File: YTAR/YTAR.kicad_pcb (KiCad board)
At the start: 6 copper layers, 50 x 50 mm, 223 parts, among them J1 STDC14, J2 CAMERA, J3 Micro_Sd, J4 FH12-40S-0.5SH(55), J5 USB_C_USB4085-GF-A, J6 IO, SW1 RESET, SW2 PICTURE, SW3 MODE, U1 STM32H750XBHx, U2 MCP2562-E-MF, U3 DS90C124, U5 TPS56339, U6 TPS56339, Y1 25MHz

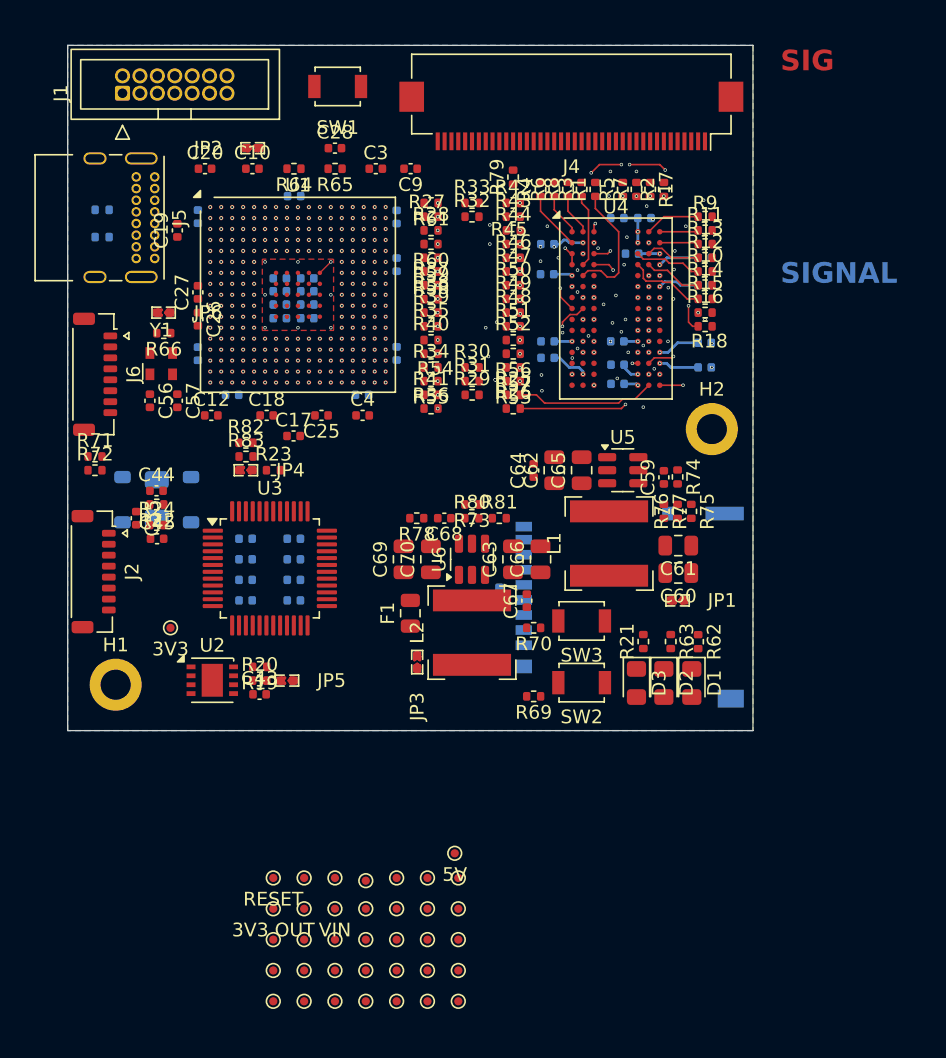
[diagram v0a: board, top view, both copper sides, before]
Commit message: routing checkpoint
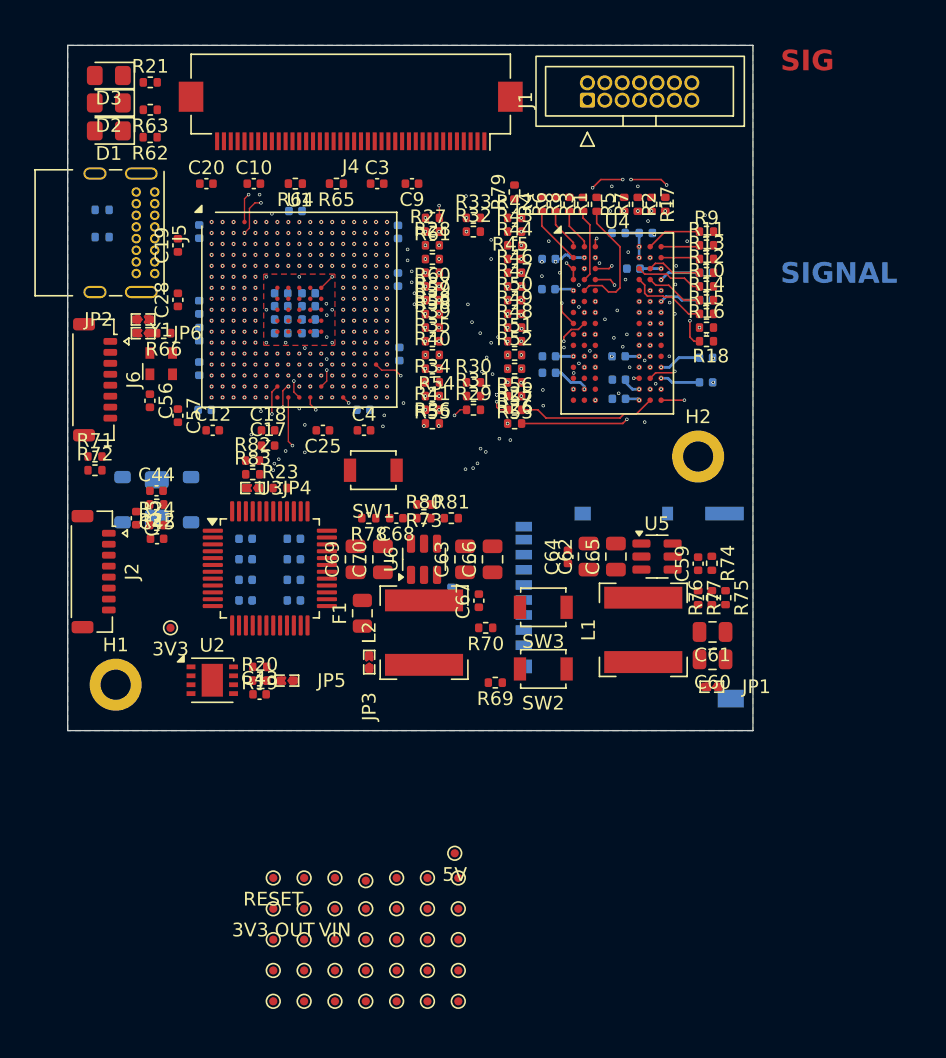
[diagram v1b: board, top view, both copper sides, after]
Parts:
- C26, C27: moved to B.Cu
- moved D3 58.7 mm to (15.0, 14.2), turned to 180 degrees
- moved D1 58.6 mm to (15.0, 18.2), turned to 180 degrees
- moved D2 58.6 mm to (15.0, 16.2), turned to 180 degrees
- moved R21 54.4 mm to (18.0, 14.7), turned to 0 degrees
- moved R62 54.3 mm to (18.0, 18.7), turned to 180 degrees
- moved R63 54.3 mm to (18.0, 16.7), turned to 180 degrees
- moved J1 33.9 mm to (49.9, 16.0)
- moved SW1 28.1 mm to (34.3, 43.0)
- moved J4 16.1 mm to (32.6, 17.1)
- moved C28 15.9 mm to (20.0, 30.6), turned to 90 degrees
- moved JP2 14.8 mm to (17.5, 32.0)
- moved C59 6.78 mm to (58.0, 49.8)
- moved C60 6.78 mm to (59.0, 56.8)
- moved C61 6.78 mm to (59.0, 54.8)
- moved C62 6.78 mm to (50.0, 49.3)
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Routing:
- net Net-(U1-PF13): track 0.00 -> 38.1 mm, vias 1 -> 6
- net Net-(U1-PF12): track 0.00 -> 35.7 mm, vias 1 -> 5
- net Net-(U1-PF11): track 0.00 -> 32.7 mm, vias 1 -> 5
- net Net-(U1-PF15): track 0.00 -> 28.0 mm, vias 1 -> 6
- net Net-(U1-PE0): track 0.00 -> 27.2 mm, vias 1 -> 4
- net Net-(U1-PG0): track 0.00 -> 27.1 mm, vias 1 -> 6
- net Net-(U1-PH5): track 0.00 -> 26.6 mm, vias 1 -> 4
- net Net-(U1-PG1): track 0.00 -> 24.3 mm, vias 1 -> 3
- net Net-(U1-PE1): track 0.00 -> 18.4 mm, vias 1 -> 3
- net Net-(U1-PG15): track 0.00 -> 14.6 mm, vias 1 -> 3
- net Net-(U1-PD15): track 0.00 -> 14.4 mm, vias 1 -> 3
- net Net-(U1-PE9): track 0.00 -> 13.7 mm, vias 1 -> 3
- net Net-(U1-PE10): track 0.00 -> 12.6 mm, vias 1 -> 4
- net Net-(U1-PD14): track 0.00 -> 12.6 mm, vias 1 -> 3
- net Net-(U1-PE8): track 0.00 -> 12.0 mm, vias 1 -> 3
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
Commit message: DRAM routed
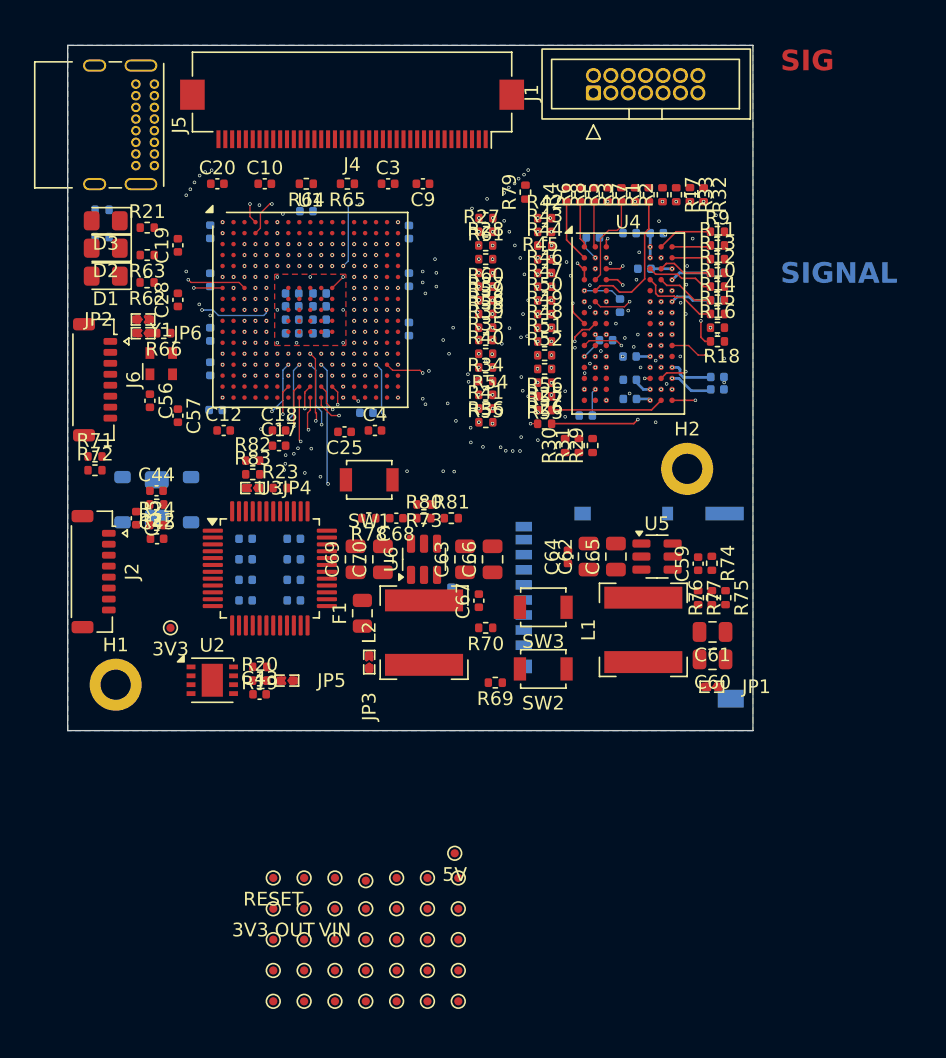
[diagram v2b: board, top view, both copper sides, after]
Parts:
- moved R32 17.0 mm to (58.4, 22.9), turned to -90 degrees
- moved R33 15.9 mm to (57.4, 22.9), turned to -90 degrees
- moved D1 10.6 mm to (14.8, 28.8)
- moved D2 10.6 mm to (14.8, 26.8)
- moved D3 10.6 mm to (14.8, 24.8)
- moved R21 10.6 mm to (17.8, 25.3)
- moved R62 10.6 mm to (17.8, 29.3)
- moved R63 10.6 mm to (17.8, 27.3)
- moved R29 9.07 mm to (50.3, 41.2), turned to 90 degrees
- moved R31 8.50 mm to (49.3, 41.2), turned to 90 degrees
- moved R30 8.12 mm to (48.3, 41.2), turned to 90 degrees
- moved J5 7.88 mm to (18.3, 14.8)
- moved C37 5.36 mm to (52.3, 31.0), turned to -90 degrees
- moved C32 4.32 mm to (51.3, 33.5), turned to 0 degrees
- moved C40 4.11 mm to (49.8, 39.0)
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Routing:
- net Net-(U1-PF4): track 0.00 -> 47.1 mm, vias 1 -> 6
- net Net-(U1-PF5): track 0.00 -> 46.0 mm, vias 2 -> 5
- net Net-(U1-PF3): track 0.00 -> 44.4 mm, vias 1 -> 6
- net Net-(U1-PF1): track 0.00 -> 39.8 mm, vias 1 -> 5
- net Net-(U1-PF2): track 0.00 -> 39.7 mm, vias 1 -> 5
- net Net-(U1-PF0): track 0.00 -> 39.1 mm, vias 1 -> 6
- net Net-(U1-PF14): track 0.00 -> 32.7 mm, vias 2 -> 6
- net Net-(U1-PE0): track 27.2 -> 2.96 mm, vias 4 -> 3
- net /NBL1: track 0.00 -> 20.4 mm, vias 0 -> 2
- net Net-(U1-PE11): track 11.3 -> 31.1 mm, vias 3 -> 5
- net Net-(U1-PE12): track 10.8 -> 30.2 mm, vias 3 -> 5
- net Net-(U1-PE1): track 18.4 -> 2.72 mm, vias 3 -> 1
- net Net-(U1-PE8): track 12.0 -> 27.5 mm, vias 3 -> 5
- net /NBL0: track 0.00 -> 14.1 mm, vias 0 -> 2
- net Net-(U1-PE10): track 12.6 -> 25.3 mm, vias 4 -> 5
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
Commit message: DRAM routed hmm
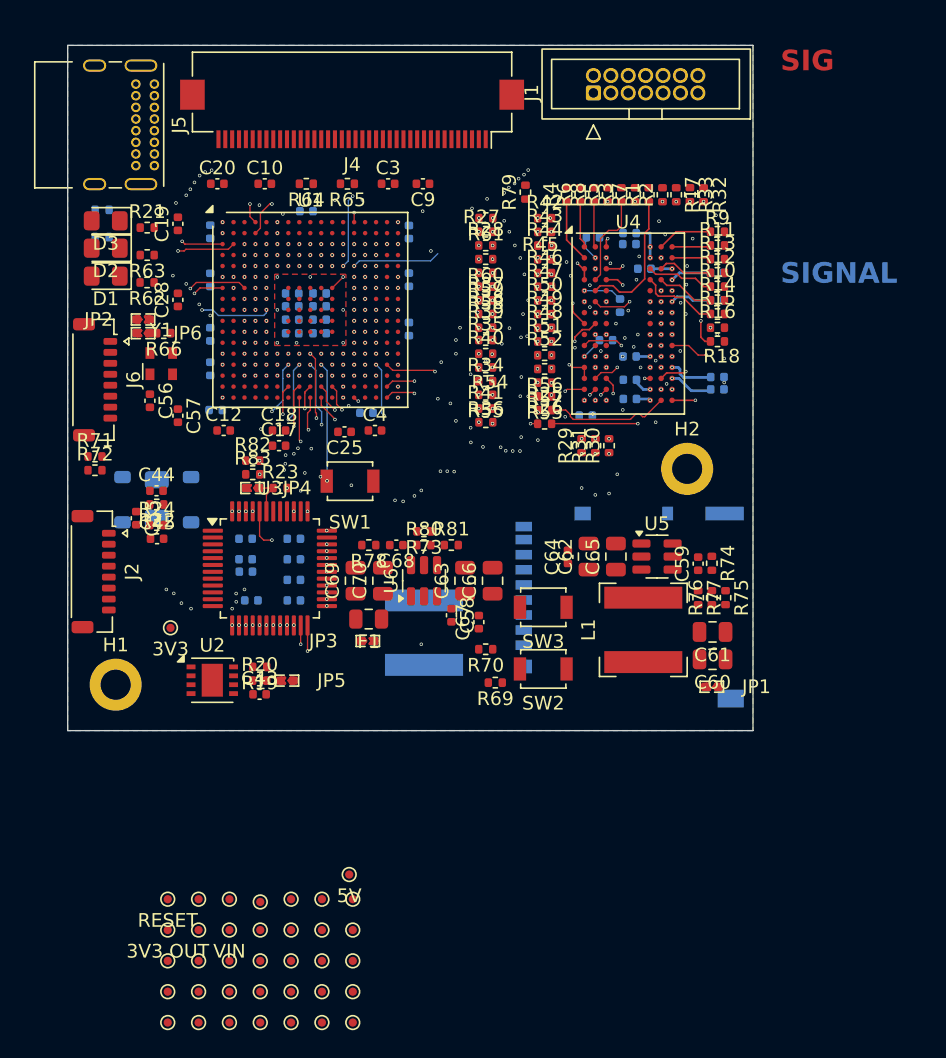
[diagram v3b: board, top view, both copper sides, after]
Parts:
- C58: moved to F.Cu
- L2: moved to B.Cu
- moved TP12 7.85 mm to (32.5, 72.5)
- moved TP33 7.85 mm to (32.8, 74.3)
- moved TP34 7.85 mm to (32.8, 76.5)
- moved TP35 7.85 mm to (32.8, 78.8)
- moved TP36 7.85 mm to (32.8, 81.0)
- moved TP37 7.85 mm to (32.8, 83.3)
- moved TP1 7.85 mm to (19.3, 74.3)
- moved TP10 7.85 mm to (21.6, 83.3)
- moved TP11 7.85 mm to (23.8, 74.3)
- moved TP14 7.85 mm to (23.8, 76.5)
- moved TP15 7.85 mm to (23.8, 78.8)
- moved TP16 7.85 mm to (23.8, 81.0)
- moved TP17 7.85 mm to (23.8, 83.3)
- moved TP18 7.85 mm to (26.1, 74.5)
- moved TP19 7.85 mm to (26.1, 76.5)
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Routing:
- net /ROUT12: track 0.00 -> 52.6 mm, vias 1 -> 6
- net /ROUT10: track 0.00 -> 45.1 mm, vias 0 -> 5
- net /ROUT9: track 0.00 -> 44.4 mm, vias 1 -> 4
- net /DQ12: track 0.00 -> 38.5 mm, vias 1 -> 5
- net /ROUT14: track 0.00 -> 36.0 mm, vias 0 -> 4
- net /ROUT13: track 0.00 -> 36.0 mm, vias 1 -> 5
- net /ROUT15: track 0.00 -> 34.4 mm, vias 0 -> 4
- net Net-(U1-PD10): track 0.00 -> 28.7 mm, vias 0 -> 4
- net Net-(U1-PD9): track 0.00 -> 28.2 mm, vias 0 -> 4
- net Net-(U1-PD8): track 0.00 -> 24.9 mm, vias 0 -> 4
- net /DES_RCLK: track 0.00 -> 12.2 mm, vias 0 -> 2
- net /DES_LOCK: track 0.00 -> 11.0 mm, vias 0 -> 2
- net /ROUT8: track 0.00 -> 8.35 mm, vias 1 -> 2
- net GND: track 3.24 -> 8.61 mm, vias 47 -> 51
- net /DQ14: track 0.00 -> 4.73 mm, vias 0 -> 2
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
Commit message: Huuuh
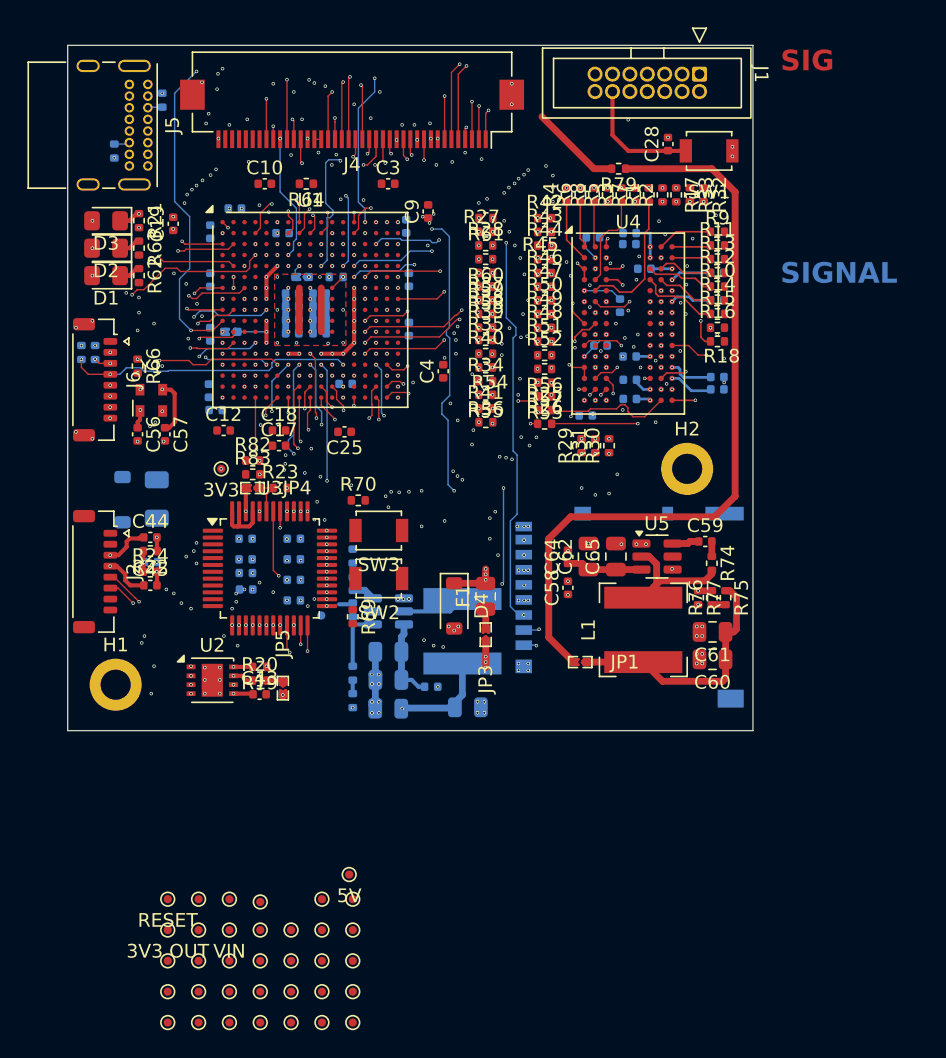
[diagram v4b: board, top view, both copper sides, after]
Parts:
- C20, C55, C63, C66, C67, C68, C69, C70, JP2, JP6, R65, R71, R72, R73, R78, R80, R81, TP23, U6: moved to B.Cu
- D4: moved to F.Cu
- moved C28 37.5 mm to (55.8, 19.2)
- moved SW1 35.6 mm to (58.8, 19.7)
- moved TP23 20.8 mm to (30.5, 53.6), turned to 180 degrees
- moved D4 20.7 mm to (40.2, 52.9)
- moved R70 14.3 mm to (33.2, 45.2), turned to 0 degrees
- moved SW2 13.7 mm to (34.7, 50.9)
- moved R73 13.4 mm to (32.8, 59.8), turned to 90 degrees
- moved SW3 13.2 mm to (34.7, 47.4)
- moved TP13 12.2 mm to (23.2, 42.9)
- moved JP2 12.0 mm to (29.1, 28.9), turned to 0 degrees
- moved R69 11.5 mm to (32.8, 53.7), turned to -90 degrees
- moved C70 11.1 mm to (41.2, 60.3), turned to 0 degrees
- moved R80 10.7 mm to (32.8, 57.8), turned to 90 degrees
- moved C66 10.5 mm to (35.4, 58.3), turned to 180 degrees
- moved JP1 9.77 mm to (49.4, 57.0)
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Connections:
- JP5 pad 1: /CAN_L -> /CAM_CAN_L
- R20 pad 1: /CAN_H -> /CAM_CAN_H
- U1 pad B17: /FD_CAN1_RX -> unconnected-(U1-PH14-PadB17)
- U1 pad D5: unconnected-(U1-PB8-PadD5) -> /FD_CAN1_RX
- U1 pad R3: unconnected-(U1-PA6-PadR3) -> /IO_AUX_1
- U1 pad T3: unconnected-(U1-PA5-PadT3) -> /IO_AUX_2
- U2 pad 1: /CAN_TX -> /FD_CAN1_TX
- U2 pad 4: /CAN_RX -> /FD_CAN1_RX
- U2 pad 6: /CAN_L -> /CAM_CAN_L
- U2 pad 7: /CAN_H -> /CAM_CAN_H
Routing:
- net /~{STM_RST}: track 0.00 -> 64.8 mm, vias 0 -> 2
- net /LCD_R5: track 0.00 -> 64.3 mm, vias 0 -> 4
- net /SD_D3: track 0.00 -> 61.9 mm, vias 0 -> 4
- net /LCD_R4: track 0.00 -> 61.7 mm, vias 0 -> 4
- net /SD_D2: track 0.00 -> 60.9 mm, vias 0 -> 4
- net +5V: track 0.00 -> 55.5 mm, vias 0 -> 1
- net /ROUT11: track 0.00 -> 53.4 mm, vias 1 -> 4
- net /LCD_R1: track 0.00 -> 51.4 mm, vias 1 -> 4
- net /LCD_R2: track 0.00 -> 51.2 mm, vias 1 -> 4
- net /FD_CAN1_RX: track 0.00 -> 44.4 mm, vias 0 -> 4
- net /LCD_R0: track 0.00 -> 44.3 mm, vias 1 -> 4
- net /SD_CMD: track 0.00 -> 41.9 mm, vias 1 -> 3
- net /JTDO/SWO: track 0.00 -> 41.9 mm, vias 1 -> 2
- net /FD_CAN1_TX: track 0.00 -> 41.5 mm, vias 1 -> 4
- net /SD_CK: track 0.00 -> 40.8 mm, vias 0 -> 6
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- removed copper zone on B.Cu, net GND

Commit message: Trud skonczon
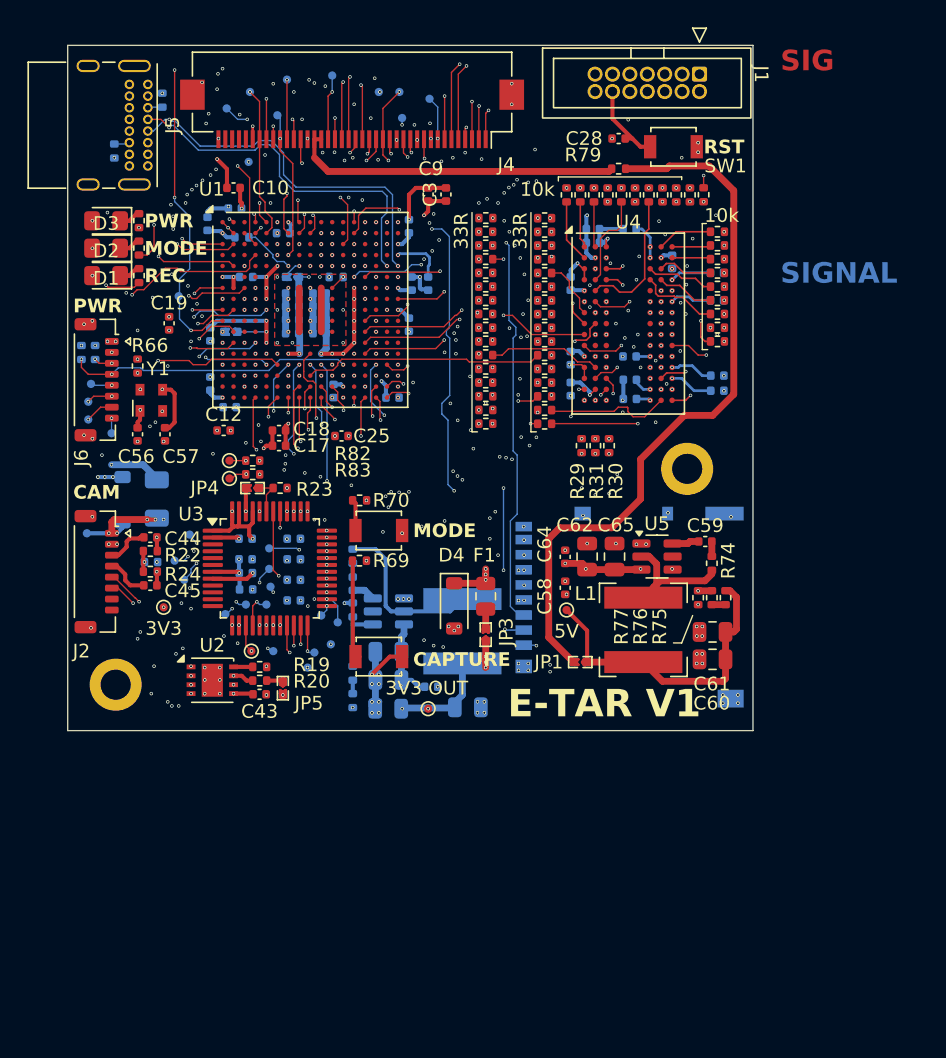
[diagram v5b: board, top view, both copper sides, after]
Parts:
- added C71: 2.2u, Capacitor_SMD:C_0402_1005Metric, B.Cu at (27.7, 25.7)
- C4, R64, TP1, TP10, TP11, TP14, TP15, TP16, TP17, TP18, TP19, TP20, TP21, TP22, TP24, TP25, TP26, TP27, TP28, TP3, TP30, TP31, TP34, TP35, TP36, TP37, TP4, TP5, TP6, TP7, TP8, TP9: moved to B.Cu
- moved TP5 70.1 mm to (31.3, 14.2), turned to 180 degrees
- moved TP4 67.8 mm to (36.2, 15.4), turned to 180 degrees
- moved TP10 67.6 mm to (36.4, 17.3), turned to 180 degrees
- moved TP3 65.7 mm to (38.4, 15.9), turned to 180 degrees
- moved TP8 64.6 mm to (28.0, 14.5), turned to 180 degrees
- moved TP9 64.2 mm to (27.3, 17.1), turned to 180 degrees
- moved TP15 63.4 mm to (25.3, 15.4), turned to 180 degrees
- moved TP7 60.0 mm to (23.6, 16.6), turned to 180 degrees
- moved TP11 59.9 mm to (34.7, 15.4), turned to 180 degrees
- moved TP6 53.9 mm to (25.2, 20.5), turned to 180 degrees
- moved TP37 46.5 mm to (15.2, 40.3), turned to 180 degrees
- moved TP36 46.0 mm to (13.5, 39.3), turned to 180 degrees
- moved TP35 45.1 mm to (13.5, 38.0), turned to 180 degrees
- moved TP34 44.2 mm to (13.7, 36.7), turned to 180 degrees
- moved TP1 44.0 mm to (20.1, 30.3), turned to 180 degrees
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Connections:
- net /IO_AUX_1 renamed /DCMI_PIXCLK
- C2 pad 1: Net-(C1-Pad1) -> Net-(C2-Pad1)
- U1 pad A2: unconnected-(U1-PI6-PadA2) -> /LED_ORANGE
- U1 pad A3: unconnected-(U1-PI5-PadA3) -> /DCMI_VSYNC
- U1 pad A4: unconnected-(U1-PI4-PadA4) -> /LED_GREEN
- U1 pad A5: unconnected-(U1-PB5-PadA5) -> /LCD_AUX_1
- U1 pad A7: Net-(C1-Pad1) -> Net-(C71-Pad1)
- U1 pad B16: unconnected-(U1-PH15-PadB16) -> /DCMI_D11
- U1 pad B17: unconnected-(U1-PH14-PadB17) -> /DCMI_D4
- U1 pad B5: unconnected-(U1-PB6-PadB5) -> /LCD_PWM
- U1 pad P13: unconnected-(U1-PH10-PadP13) -> /DCMI_D1
- U1 pad P14: unconnected-(U1-PH11-PadP14) -> /DCMI_D2
- U1 pad R14: unconnected-(U1-PH12-PadR14) -> /DCMI_D3
- U1 pad R15: unconnected-(U1-PD11-PadR15) -> /SD_DET_A
- U1 pad T14: unconnected-(U1-PB12-PadT14) -> /SW_MODE
- U1 pad U11: Net-(C1-Pad1) -> Net-(C2-Pad1)
- U1 pad U14: unconnected-(U1-PB13-PadU14) -> /SW_PICTURE
- U1 pad U3: unconnected-(U1-PA4-PadU3) -> /DCMI_HSYNC
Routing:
- net +12V_CAM: track 11.5 -> 79.5 mm, vias 0 -> 15
- net Net-(U1-PE0): track 2.96 -> 45.6 mm, vias 3 -> 2
- net Net-(U1-PE1): track 2.72 -> 39.4 mm, vias 1 -> 4
- net GND: track 29.2 -> 65.0 mm, vias 155 -> 189
- net /SD_DET_A: track 0.00 -> 33.8 mm, vias 0 -> 3
- net +3.3V: track 56.5 -> 84.3 mm, vias 77 -> 85
- net /D-: track 1.70 -> 28.8 mm, vias 0 -> 2
- net /D+: track 1.94 -> 28.5 mm, vias 0 -> 2
- net /LED_GREEN: track 0.00 -> 19.4 mm, vias 0 -> 3
- net Net-(J4-Pin_25): track 7.16 -> 24.0 mm, vias 1 -> 0
- net /ROUT10: track 43.9 -> 59.1 mm
- net Net-(J6-Pin_1): track 0.00 -> 13.9 mm, vias 0 -> 4
- net /SW_PICTURE: track 0.00 -> 12.3 mm, vias 0 -> 2
- net Net-(U1-PF15): track 28.6 -> 17.5 mm, vias 4 -> 0
- net /LCD_PWM: track 0.00 -> 11.1 mm, vias 0 -> 1
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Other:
- board text added: "10k"
- board text added: "33R"
- board text added: "CAM"
- board text added: "CAPTURE"
- board text added: "E-TAR V1"
- board text added: "MODE"
- board text added: "REC"
- board text added: "RST"
